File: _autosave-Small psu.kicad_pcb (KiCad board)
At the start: 2 copper layers, 78 x 49 mm, 38 parts, among them J1 VDC-in, J2 V out, J3 V select sw, J4 reset sw, Q1 FQP27P06, Q2 BC547, U1 LM321, U2 LM317T, U3 LM317T, U4 LM311N, U5 LM358

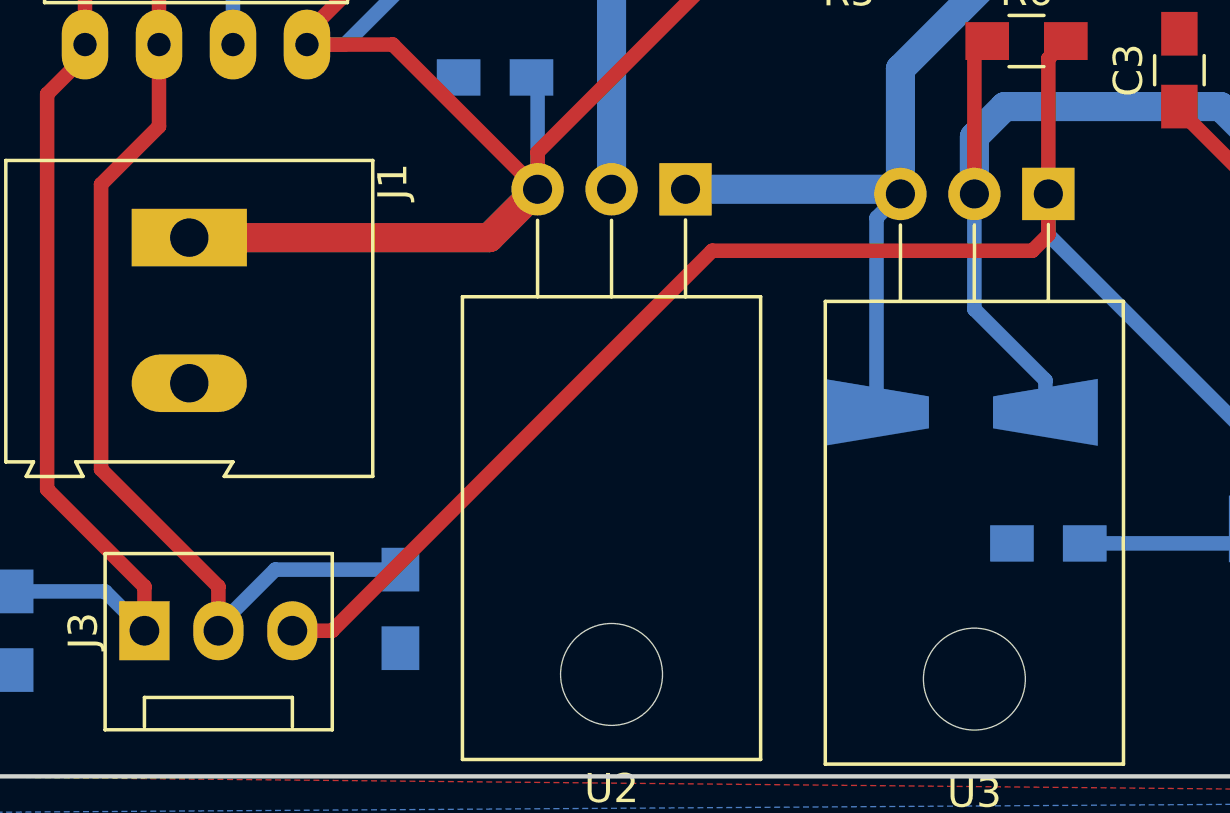
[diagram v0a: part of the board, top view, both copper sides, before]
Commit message: Add files via upload
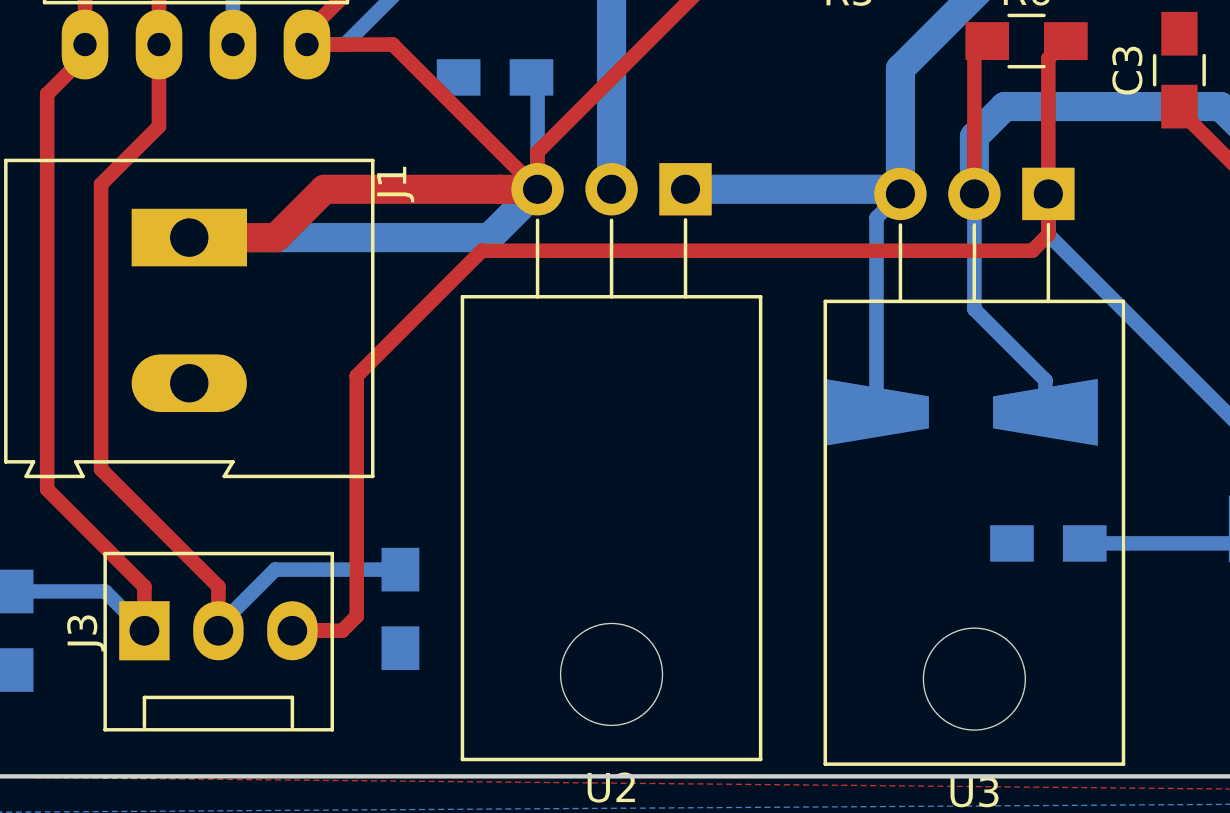
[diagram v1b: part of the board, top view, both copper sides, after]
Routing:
- net Net-(C2-Pad1): track 60.3 -> 66.5 mm
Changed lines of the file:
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@@
     (thickness 1.6)
     (drawings 6)
-    (tracks 188)
+    (tracks 193)
     (zones 0)
     (modules 38)
@@
     (visible_elements 7FFFEFFF)
     (pcbplotparams
-      (layerselection 0x01000_fffffffe)
+      (layerselection 0x01000_ffffffff)
       (usegerberextensions false)
       (excludeedgelayer true)
@@
   (segment (start 172.34 57.88) (end 175.5 61.04) (width 0.5) (layer F.Cu) (net 1))
   (segment (start 175.5 61.04) (end 175.5 62.75) (width 0.5) (layer F.Cu) (net 1) (status 20))
+  (segment (start 135.187208 80.34) (end 136.46 80.34) (width 1) (layer F.Cu) (net 2))
+  (segment (start 129.14 80.34) (end 135.187208 80.34) (width 1) (layer F.Cu) (net 2))
+  (segment (start 127.48 82) (end 129.14 80.34) (width 1) (layer F.Cu) (net 2))
+  (segment (start 124.5 82) (end 127.48 82) (width 1) (layer F.Cu) (net 2))
   (segment (start 178.925 63.75) (end 177.425 65.25) (width 0.5) (layer F.Cu) (net 2))
   (segment (start 179.75 59.5) (end 179.75 63.75) (width 0.4) (layer F.Cu) (net 2) (status 30))
@@
   (segment (start 128.54 74.97) (end 131.51 72) (width 0.5) (layer F.Cu) (net 2) (status 10))
   (segment (start 131.51 72) (end 132.5 72) (width 0.5) (layer F.Cu) (net 2) (status 20))
-  (segment (start 134.8 82) (end 136.46 80.34) (width 1) (layer F.Cu) (net 2) (status 20))
-  (segment (start 124.5 82) (end 134.8 82) (width 1) (layer F.Cu) (net 2) (status 10))
   (segment (start 131.75 70.85) (end 131.75 73.46) (width 0.5) (layer B.Cu) (net 2) (status 10))
   (segment (start 131.75 73.46) (end 129.84 75.37) (width 0.5) (layer B.Cu) (net 2))
@@
   (segment (start 162.5 73.15) (end 166.65 73.15) (width 0.5) (layer B.Cu) (net 12) (status 30))
   (segment (start 166.65 73.15) (end 166.73 73.23) (width 0.5) (layer B.Cu) (net 12) (status 30))
-  (segment (start 154 81.9) (end 154 80.5) (width 0.5) (layer F.Cu) (net 13) (status 20))
-  (segment (start 153.449999 82.450001) (end 154 81.9) (width 0.5) (layer F.Cu) (net 13))
-  (segment (start 142.454999 82.450001) (end 153.449999 82.450001) (width 0.5) (layer F.Cu) (net 13))
-  (segment (start 129.405 95.5) (end 142.454999 82.450001) (width 0.5) (layer F.Cu) (net 13))
+  (segment (start 154 80.5) (end 154 81.9) (width 0.5) (layer F.Cu) (net 13))
+  (segment (start 154 81.9) (end 153.449999 82.450001) (width 0.5) (layer F.Cu) (net 13))
+  (segment (start 153.449999 82.450001) (end 134.549999 82.450001) (width 0.5) (layer F.Cu) (net 13))
+  (segment (start 134.549999 82.450001) (end 130.25 86.75) (width 0.5) (layer F.Cu) (net 13))
+  (segment (start 130.25 95) (end 129.75 95.5) (width 0.5) (layer F.Cu) (net 13))
+  (segment (start 130.25 86.75) (end 130.25 95) (width 0.5) (layer F.Cu) (net 13))
+  (segment (start 129.75 95.5) (end 128.04 95.5) (width 0.5) (layer F.Cu) (net 13))
   (segment (start 128.04 95.5) (end 129.405 95.5) (width 0.5) (layer F.Cu) (net 13) (status 10))
   (segment (start 154 80.5) (end 154 75.85) (width 0.5) (layer F.Cu) (net 13) (status 30))
